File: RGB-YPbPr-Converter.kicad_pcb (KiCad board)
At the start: 2 copper layers, 54.5 x 35 mm, 43 parts, among them J1 RGB, J2 Component, J3 PWR, Q1 Q_NPN_BEC, Q2 Q_NPN_BEC, Q3 Q_NPN_BEC, U1 LMV793MFX, U2 LT6550, U3 ICL7660

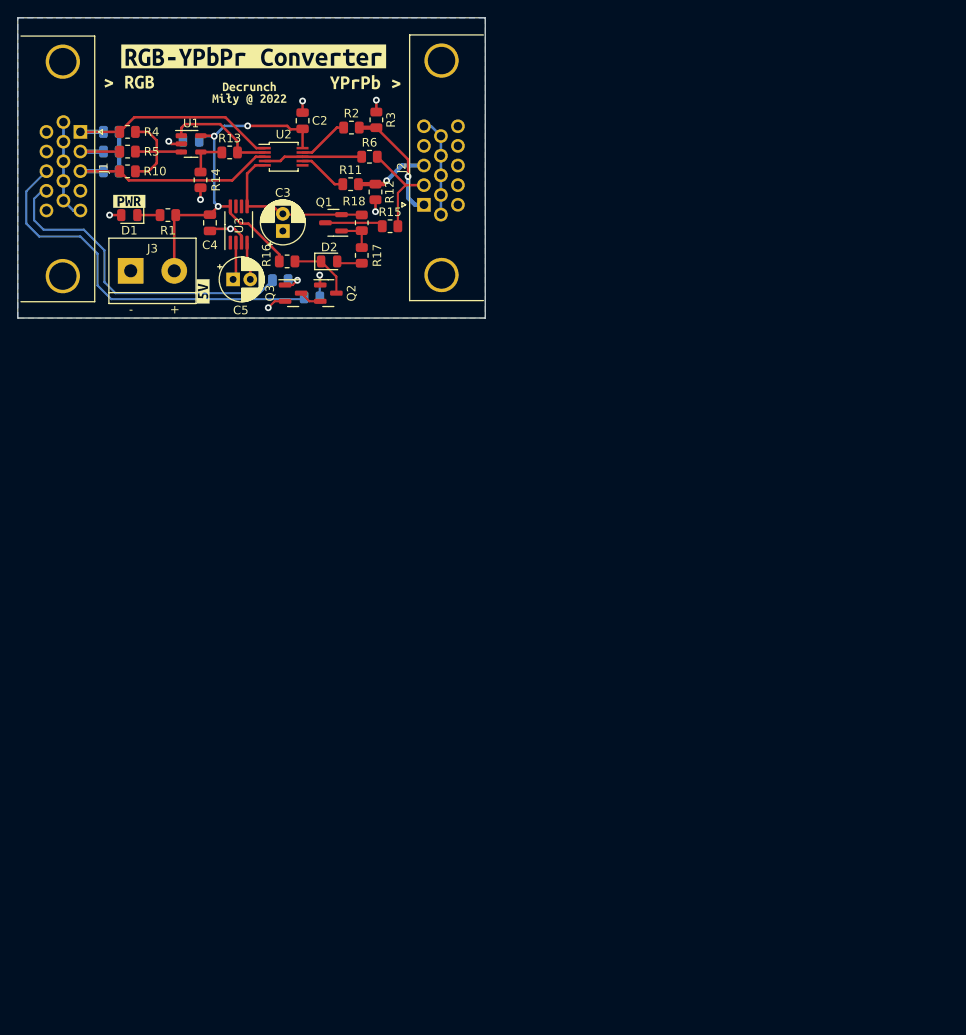
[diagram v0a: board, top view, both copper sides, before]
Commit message: finished board
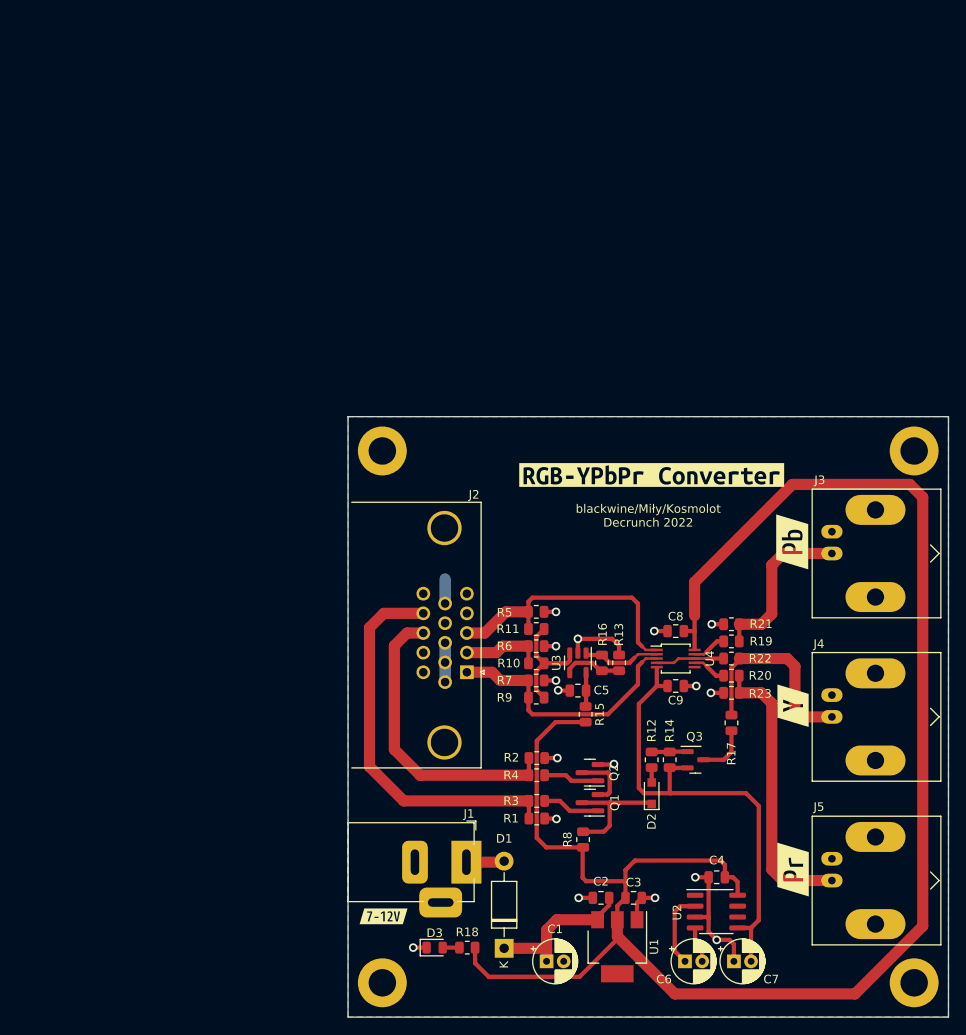
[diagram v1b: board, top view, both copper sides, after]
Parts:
- removed the J2 at (108.8, 75.3)
- removed kibuzzard-63377BCB: G***, kibuzzard-63377BCB
- removed kibuzzard-63377BDE: G***, kibuzzard-63377BDE
- removed kibuzzard-63377C0B: G***, kibuzzard-63377C0B
- removed kibuzzard-63377C27: G***, kibuzzard-63377C27
- removed kibuzzard-63377CAE: G***, kibuzzard-63377CAE
- removed kibuzzard-63377D38: G***, kibuzzard-63377D38
- added C1: 10u/16V, Capacitor_THT:CP_Radial_D5.0mm_P2.00mm, F.Cu at (123.1, 163.5)
- added C2: 100n, Capacitor_SMD:C_0805_2012Metric, F.Cu at (129.5, 156.1)
- added C3: 100n, Capacitor_SMD:C_0805_2012Metric, F.Cu at (133.3, 156.1)
- added C9: 100n, Capacitor_SMD:C_0805_2012Metric, F.Cu at (138.2, 131.4)
- added D1: 1N4001, Diode_THT:D_DO-41_SOD81_P10.16mm_Horizontal, F.Cu at (118.2, 162.0)
- added H1: DNP, MountingHole:MountingHole_3.2mm_M3_ISO7380_Pad, F.Cu at (104.0, 104.0)
- added H2: DNP, MountingHole:MountingHole_3.2mm_M3_ISO7380_Pad, F.Cu at (166.0, 104.0)
- added H3: DNP, MountingHole:MountingHole_3.2mm_M3_ISO7380_Pad, F.Cu at (104.0, 166.0)
- added H4: DNP, MountingHole:MountingHole_3.2mm_M3_ISO7380_Pad, F.Cu at (166.0, 166.0)
- added J1: Barrel Jack 5.5/2.1, Connector_BarrelJack:BarrelJack_Horizontal, F.Cu at (113.8, 151.9)
- added J4: BNC 75 Ohm, Connector_Coaxial:BNC_Amphenol_B6252HB-NPP3G-50_Horizontal, F.Cu at (156.4, 135.0)
- added J5: BNC 75 Ohm, Connector_Coaxial:BNC_Amphenol_B6252HB-NPP3G-50_Horizontal, F.Cu at (156.4, 154.1)
- added R1: 75, Resistor_SMD:R_0805_2012Metric, F.Cu at (122.0, 146.8)
- added R15: 0R, Resistor_SMD:R_0805_2012Metric, F.Cu at (127.7, 134.7)
- added R2: 75, Resistor_SMD:R_0805_2012Metric, F.Cu at (122.0, 139.8)
- added U1: 1117-5.0, Package_TO_SOT_SMD:SOT-223, F.Cu at (131.4, 161.8)
- added kibuzzard-633F44A8: G***, kibuzzard-633F44A8, F.Cu at (151.9, 152.8)
- added kibuzzard-633F44BA: G***, kibuzzard-633F44BA, F.Cu at (151.8, 114.6)
- added kibuzzard-633F44C9: G***, kibuzzard-633F44C9, F.Cu at (151.9, 133.7)
- added kibuzzard-633F4DF1: G***, kibuzzard-633F4DF1, F.Cu at (104.1, 158.3)
- C5: renamed from C1; moved to F.Cu
- C6: renamed from C5; value 10u -> 10u/16V
- C7: renamed from C3; value 10u -> 10u/16V
- D2: footprint Diode_SMD:D_0805_2012Metric -> Diode_SMD:D_SOD-323_HandSoldering
- J2: renamed from J1; value RGB -> D-Sub HD15 Female; footprint Connector_Dsub:DSUB-15-HD_Male_Horizontal_P2.29x1.98mm_EdgePinOffset3.03mm_Housed_MountingHolesOffset4.94mm -> lib:ICD15S13E4GV00LF
- J3: value PWR -> BNC 75 Ohm; footprint TerminalBlock:TerminalBlock_bornier-2_P5.08mm -> Connector_Coaxial:BNC_Amphenol_B6252HB-NPP3G-50_Horizontal
- R3: renamed from R20; moved to F.Cu
- R4: renamed from R19; moved to F.Cu
- R5: renamed from R7; moved to F.Cu
- R6: renamed from R8; moved to F.Cu
- R7: renamed from R9; moved to F.Cu
- U2: renamed from U3; footprint Package_SO:MSOP-8_3x3mm_P0.65mm -> Package_SO:SOIC-8_3.9x4.9mm_P1.27mm
- moved C7 100.1 mm to (145.0, 163.5), turned to 0 degrees
- moved U2 97.6 mm to (142.9, 157.7), turned to 0 degrees
- moved C4 96.5 mm to (143.0, 153.7), turned to 180 degrees
- moved C6 95.4 mm to (139.3, 163.5)
- moved D3 92.5 mm to (110.1, 161.9), turned to 0 degrees
- moved R18 92.3 mm to (113.9, 161.9), turned to 0 degrees
- moved J3 88.1 mm to (156.4, 116.0), turned to -90 degrees
- moved R9 81.4 mm to (121.9, 132.8)
- moved R7 80.9 mm to (121.9, 130.8)
- moved R23 78.6 mm to (144.7, 132.2), turned to 180 degrees
- moved C5 78.4 mm to (126.8, 131.9)
- moved R10 76.3 mm to (121.9, 128.8)
- moved R6 76.0 mm to (121.9, 126.8)
- moved R8 75.7 mm to (127.4, 149.3), turned to 90 degrees
- moved Q3 75.5 mm to (140.5, 140.0), turned to 0 degrees
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- renumbered C2 to C8, D1 to D3, Q2 to Q1, Q3 to Q2, Q1 to Q3, R5 to R10, R10 to R11, R17 to R12, R14 to R13, R18 to R14, R13 to R16, R15 to R17, R1 to R18, R2 to R19, R11 to R20, R12 to R21, R6 to R22, R3 to R23, R16 to R8, R4 to R9, U1 to U3, U2 to U4
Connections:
- net /Y_FB renamed /Y_OUT
- net Net-(C5-Pad1) renamed /CAP+
- net Net-(C5-Pad2) renamed /CAP-
- net Net-(R10-Pad2) renamed /YSUM
- net Net-(R11-Pad1) renamed /Pr_OUT
- net Net-(R13-Pad1) renamed /FB
- net Net-(R13-Pad2) renamed /YAMP
- net Net-(R2-Pad1) renamed /Pb_OUT
- C5 pad 1: +5V -> /+5VAMP
- D3 pad 1: Net-(D1-Pad1) -> GND
- D3 pad 2: GND -> Net-(D3-Pad2)
- J2 pad 9: GND -> unconnected-(J2-Pad9)
- J3 pad 1: GND -> /Pb
- J3 pad 2: +5V -> GND
- Q1 pad 1: Net-(Q2-Pad1) -> /V_R
- Q2 pad 1: Net-(Q3-Pad1) (its old number) -> /H_R
- R18 pad 1: +5V -> Net-(D3-Pad2)
- R18 pad 2: Net-(D1-Pad1) -> +5V
- R19 pad 2: /Pr -> /Pb
- R20 pad 2: /Pb -> /Pr
- R3 pad 2: Net-(Q3-Pad1) (its old number) -> /V_R
- R4 pad 2: Net-(Q2-Pad1) -> /H_R
- U3 pad 5: +5V -> /+5VAMP
- U4 pad 1: /R -> /B
- U4 pad 3: /B -> /R
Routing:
- net +5V: track 47.7 -> 213.4 mm, vias 3 -> 0
- net -5V: track 20.1 -> 56.1 mm
- net /VIND: track 0.00 -> 19.7 mm
- net /Pr: track 13.9 -> 33.1 mm, vias 1 -> 0
- net /Y: track 12.0 -> 23.7 mm
- net /Pb: track 8.54 -> 19.6 mm, vias 1 -> 0
- net GND: track 43.5 -> 54.1 mm, vias 8 -> 17
- net /H_SYNC: track 45.4 -> 34.9 mm
- net /V_SYNC: track 38.4 -> 45.3 mm
- net Net-(D2-Pad1): track 7.49 -> 14.3 mm
- net /V_R: track 0.00 -> 6.70 mm
- net /H_R: track 0.00 -> 6.49 mm
- net /B: track 25.7 -> 31.6 mm
- net /CAP+: track 4.42 -> 8.94 mm
- net /VIN: track 0.00 -> 4.45 mm
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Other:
- board size 54.5 x 35 mm -> 70 x 70 mm
- board text added: "Transmission line geometry: h = 1.55mm Er = 4.5 (JLCPCB 2-layer) Copper = 35um (1oz) w = 1.3mm Zo = 75 Ohm Calculated using Saturn PCB Toolkit."
- board text added: "blackwine/Miły/Kosmolot Decrunch 2022"
- board text removed: "+"
- board text removed: "-"
- board text removed: "JLCJLCJLC"
